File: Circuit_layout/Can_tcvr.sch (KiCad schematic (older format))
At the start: 4 parts, among them U10 MCP2551-I/SN

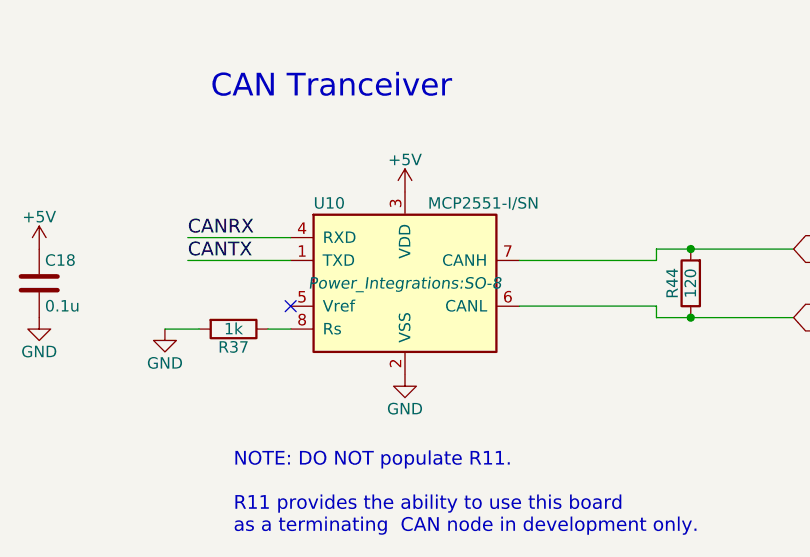
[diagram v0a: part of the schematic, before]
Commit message: changes before presentation
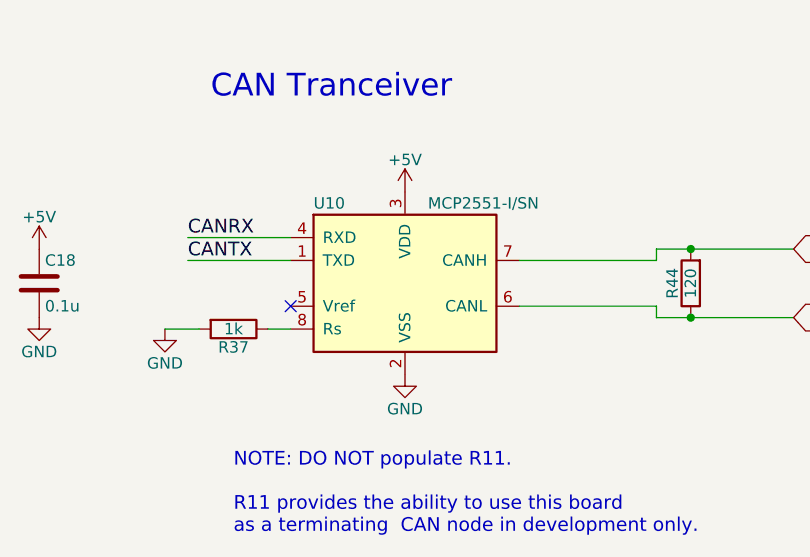
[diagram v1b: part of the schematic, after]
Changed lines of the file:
@@
 LIBS:xilinx
 LIBS:Zilog
+LIBS:pacman-main-cache
 LIBS:bss84
 LIBS:+10v
@@
 $Descr A4 11693 8268
 encoding utf-8
-Sheet 2 7
+Sheet 7 7
 Title "Tractive System Interface"
 Date ""
@@
 F 0 "U10" H 5000 4300 50  0000 L CNN
 F 1 "MCP2551-I/SN" H 5500 4300 50  0000 L CNN
-F 2 "Power_Integrations:SO-8" H 5400 3950 50  0000 C CIN
+F 2 "Power_Integrations:SO-8" H 5400 3950 50  0001 C CIN
 F 3 "" H 5400 3950 50  0000 C CNN
 F 4 "MCP2551-I/SN-ND" H 5400 3950 60  0001 C CNN "DigiKey P/N"
@@
 CANL
 $Comp
-L GND #PWR021
+L GND #PWR0122
 U 1 1 58A63637
 P 5400 4350
-F 0 "#PWR021" H 5400 4100 50  0001 C CNN
+F 0 "#PWR0122" H 5400 4100 50  0001 C CNN
 F 1 "GND" H 5400 4200 50  0000 C CNN
 F 2 "" H 5400 4350 50  0000 C CNN
@@
 $EndComp
 $Comp
-L GND #PWR022
+L GND #PWR0123
 U 1 1 58A6364F
 P 4350 4150
-F 0 "#PWR022" H 4350 3900 50  0001 C CNN
+F 0 "#PWR0123" H 4350 3900 50  0001 C CNN
 F 1 "GND" H 4350 4000 50  0000 C CNN
 F 2 "" H 4350 4150 50  0000 C CNN
@@
 	4800 4150 4900 4150
 $Comp
-L +5V #PWR023
+L +5V #PWR0124
 U 1 1 58A636CC
 P 5400 3550
-F 0 "#PWR023" H 5400 3400 50  0001 C CNN
+F 0 "#PWR0124" H 5400 3400 50  0001 C CNN
 F 1 "+5V" H 5400 3690 50  0000 C CNN
 F 2 "" H 5400 3550 50  0000 C CNN
@@
 $EndComp
 $Comp
-L +5V #PWR024
+L +5V #PWR0125
 U 1 1 58A636E7
 P 3800 3800
-F 0 "#PWR024" H 3800 3650 50  0001 C CNN
+F 0 "#PWR0125" H 3800 3650 50  0001 C CNN
 F 1 "+5V" H 3800 3940 50  0000 C CNN
 F 2 "" H 3800 3800 50  0000 C CNN
@@
 $EndComp
 $Comp
-L GND #PWR025
+L GND #PWR0126
 U 1 1 58A636FB
 P 3800 4100
-F 0 "#PWR025" H 3800 3850 50  0001 C CNN
+F 0 "#PWR0126" H 3800 3850 50  0001 C CNN
 F 1 "GND" H 3800 3950 50  0000 C CNN
 F 2 "" H 3800 4100 50  0000 C CNN
